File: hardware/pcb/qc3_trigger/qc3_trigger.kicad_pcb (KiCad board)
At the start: 2 copper layers, 12 parts, among them J1 USB_B_Micro, J2 Vout, U1 AMS1117-5.0, U2 ATtiny85V-10SU

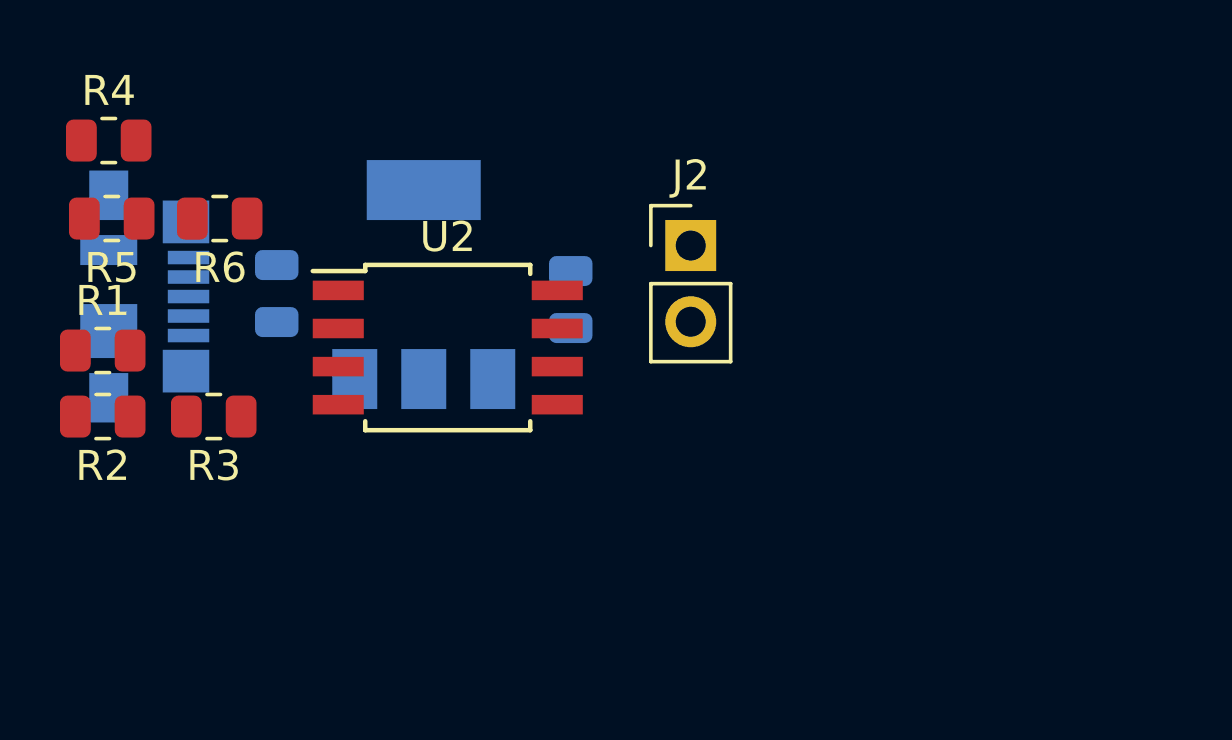
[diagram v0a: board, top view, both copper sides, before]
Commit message: наброски разводки и компановки на плате
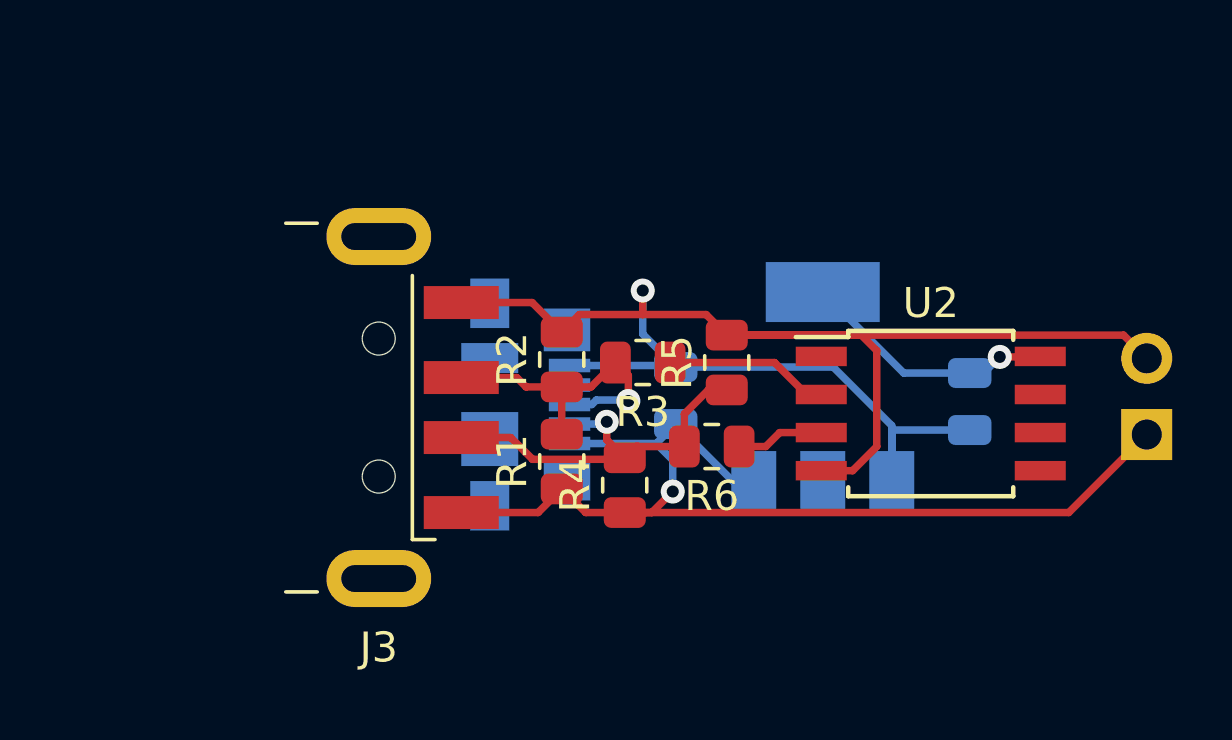
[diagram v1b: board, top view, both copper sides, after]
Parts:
- added J3: USB_A, Connector_USB:USB_A_CNCTech_1001-011-01101_Horizontal, F.Cu at (54.4, 108.4)
- J2: moved to B.Cu
- moved R5 21.1 mm to (72.9, 106.9), turned to 90 degrees
- moved R4 20.7 mm to (69.5, 111.0), turned to 90 degrees
- moved R6 18.1 mm to (72.4, 109.7)
- moved J2 16.5 mm to (86.9, 109.3)
- moved U2 16.2 mm to (79.7, 108.6)
- moved R1 15.7 mm to (67.4, 110.2), turned to 90 degrees
- moved R2 15.4 mm to (67.4, 106.8), turned to 90 degrees
- moved R3 14.4 mm to (70.1, 106.9)
- moved C1 13.7 mm to (71.2, 108.0)
- moved C2 13.7 mm to (81.0, 108.2)
- moved U1 13.7 mm to (76.1, 107.7)
- moved J1 13.2 mm to (66.2, 108.3)
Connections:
- U2 pad 2: Net-(R6-Pad1) -> Net-(R3-Pad1)
- U2 pad 3: Net-(R3-Pad1) -> Net-(R6-Pad1)
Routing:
- net GND: track 0.00 -> 56.3 mm, vias 0 -> 1
- net +5V: track 0.00 -> 36.2 mm, vias 0 -> 1
- net Net-(J1-Pad2): track 0.00 -> 13.5 mm, vias 0 -> 1
- net Net-(J1-Pad3): track 0.00 -> 10.7 mm, vias 0 -> 1
- net Net-(C2-Pad1): track 0.00 -> 8.60 mm, vias 0 -> 1
- net Net-(R3-Pad1): track 0.00 -> 5.48 mm
- net Net-(R6-Pad1): track 0.00 -> 2.93 mm
